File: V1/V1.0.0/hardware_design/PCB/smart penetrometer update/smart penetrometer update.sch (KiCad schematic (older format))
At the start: 34 parts, among them J1 XLR3_Switched, J2 Conn_01x11_Female, U2 DS3231M, U3 Battery_Input, U4 4023, U5 ADS1115IDGS, U6 3v3_Voltage_Regulator, U7 Solar_Input

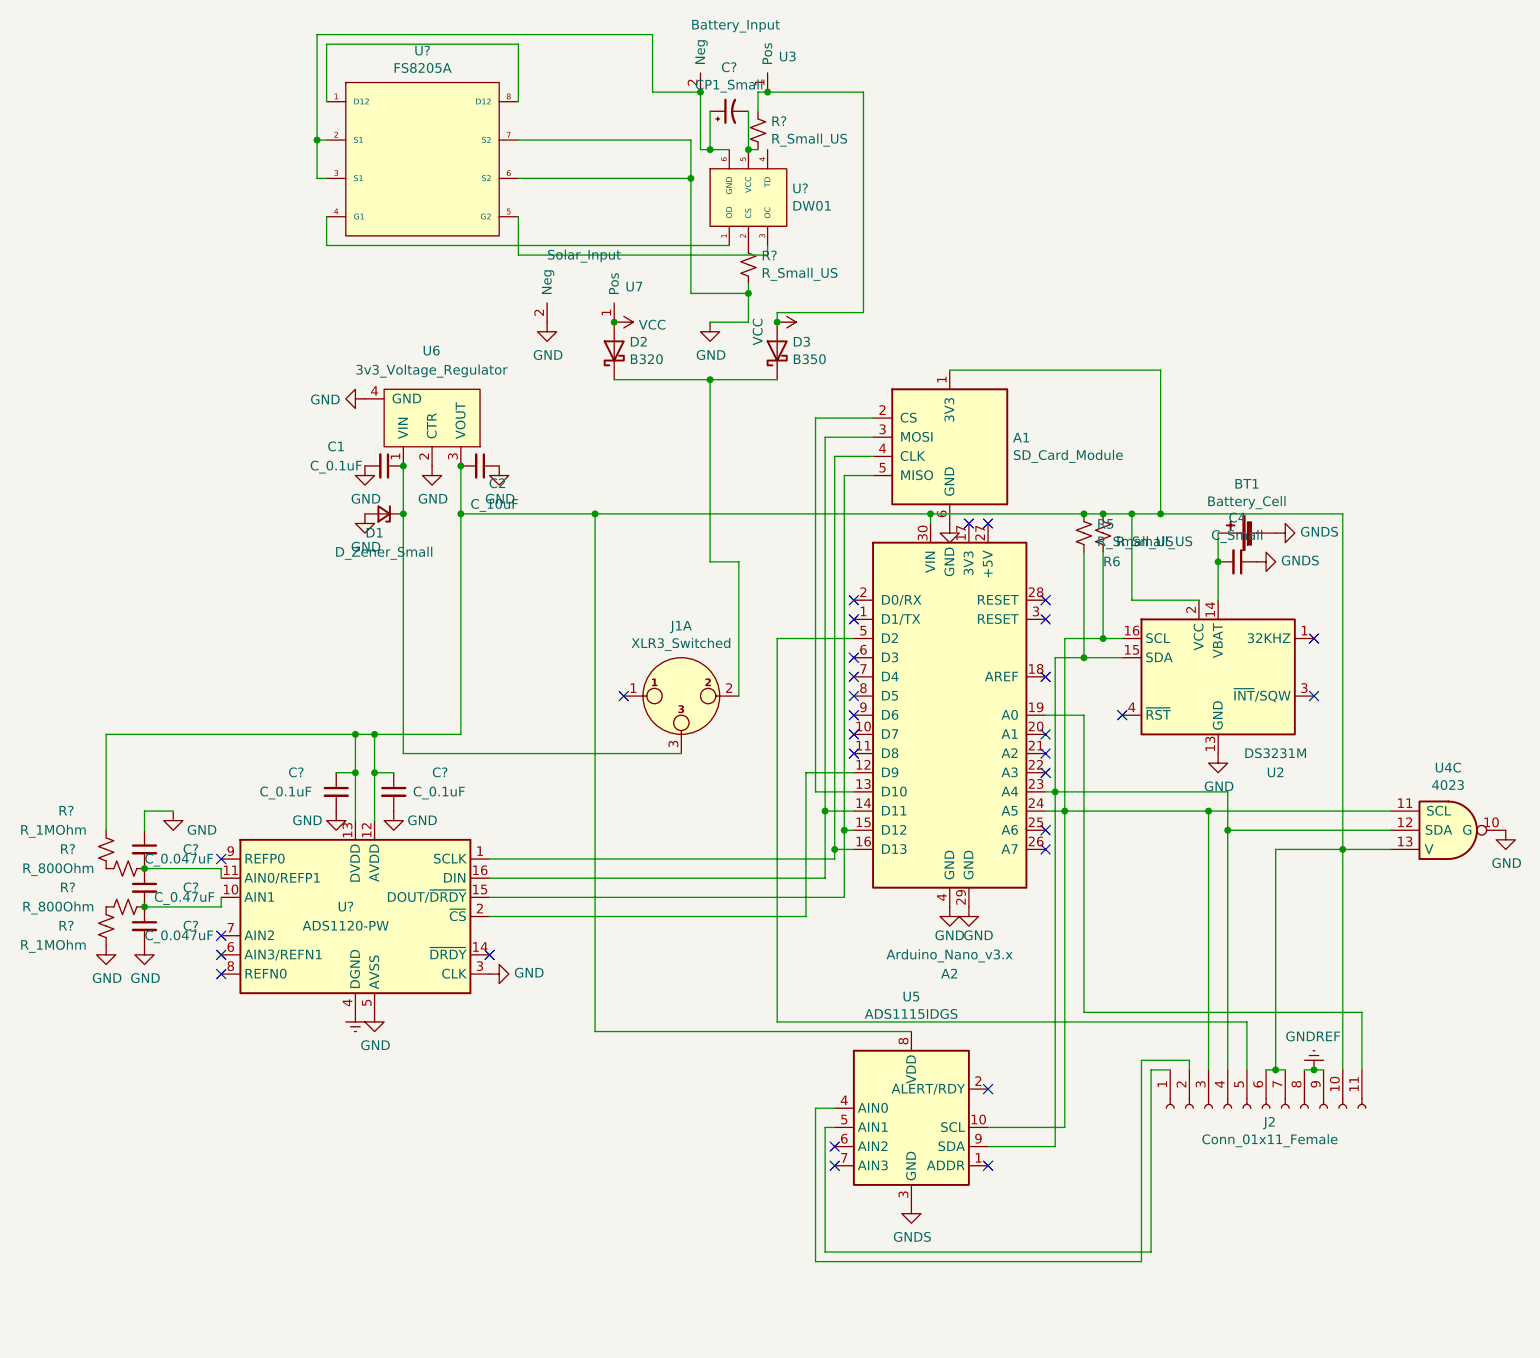
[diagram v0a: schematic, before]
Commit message: SCHEMATIC UPDAYE
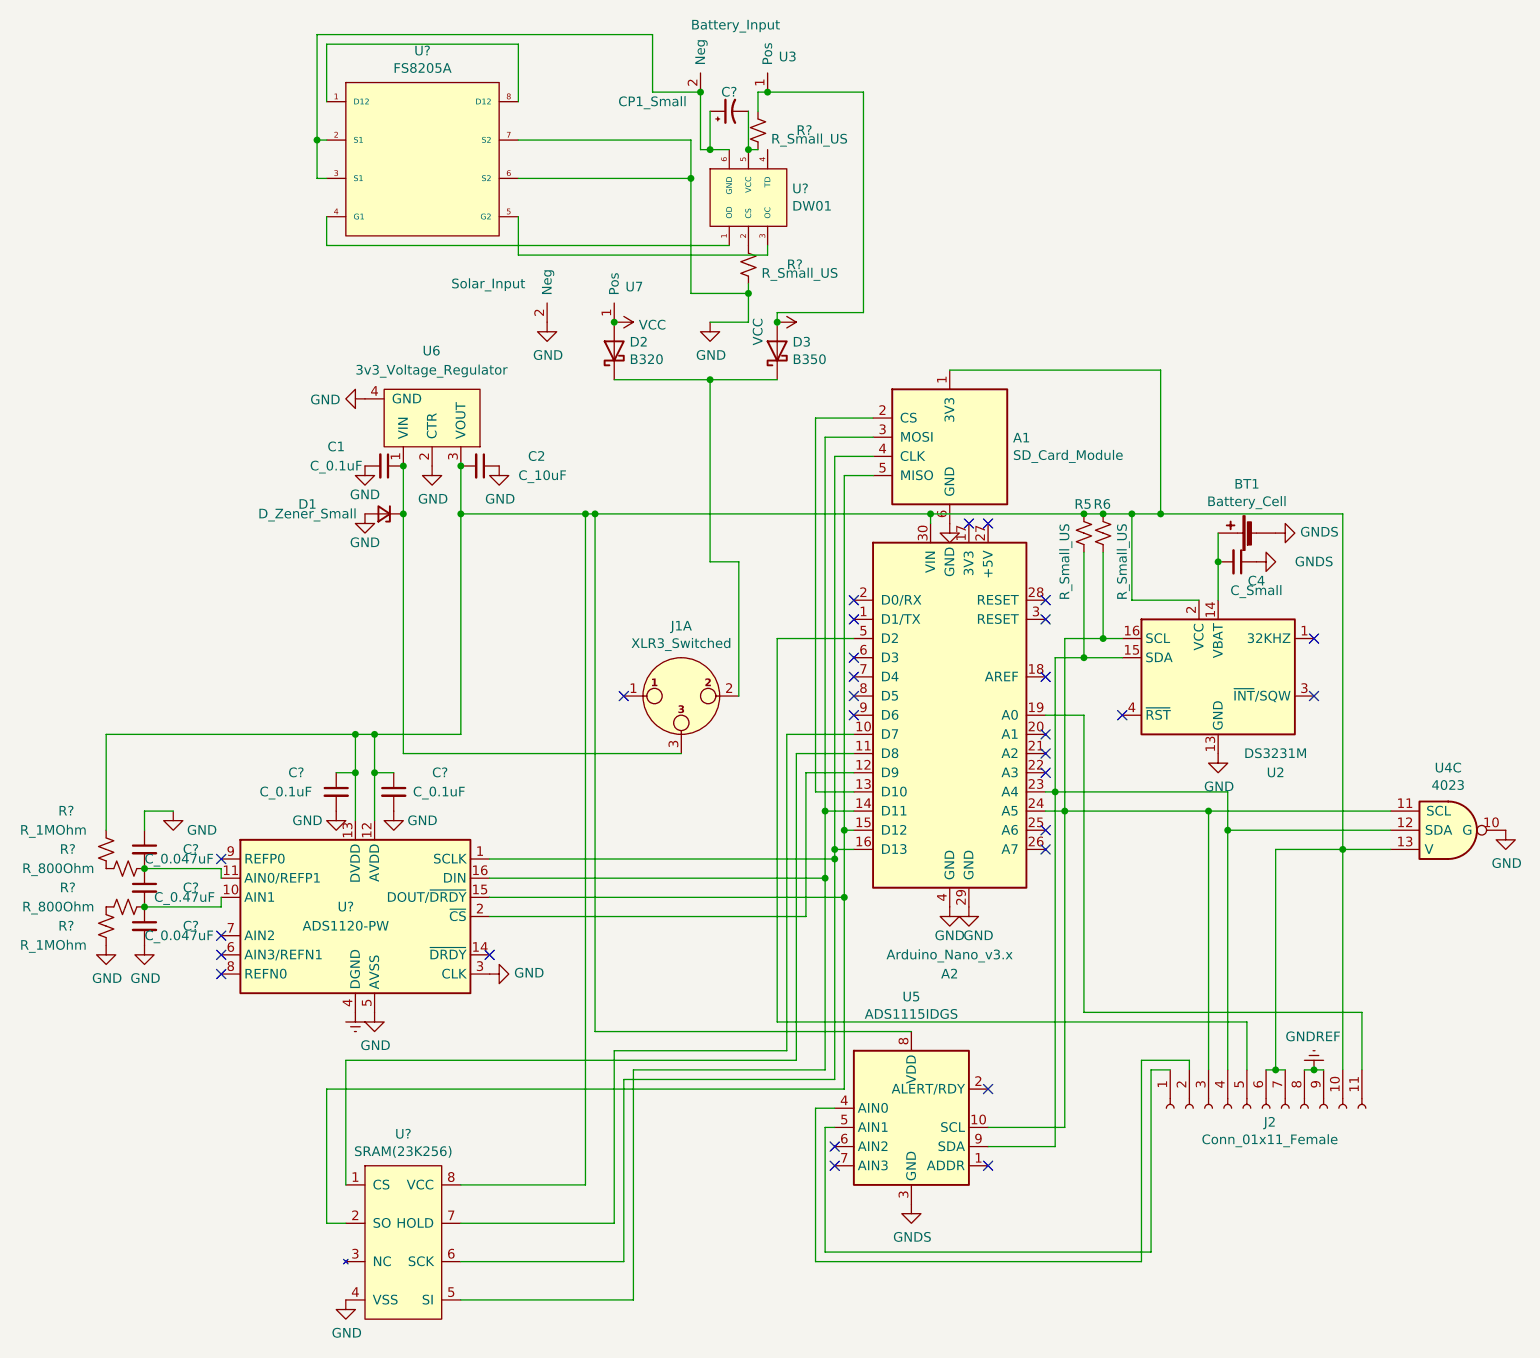
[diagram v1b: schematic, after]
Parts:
- added U?: SRAM(23K256), symbol smart-penetrometer-update-rescue:SRAM(23K256)
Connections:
- net GND: now also U?.4 (VSS)
- net at A2.10 (D7): now also U?.7 (HOLD)
- net at A2.11 (D8): now also U?.1 (CS)
- net at A1.3 (MOSI), A2.14 (D11), U?.16 (DIN): now also U?.5 (SI)
- net at A1.5 (MISO), A2.15 (D12), U?.15 (DOUT/~DRDY): now also U?.2 (SO)
- net at A1.4 (CLK), A2.16 (D13), U?.1 (SCLK): now also U?.6 (SCK)
- net at A1.1 (3V3), A2.30 (VIN), C2.2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: now also U?.8 (VCC)
- no-connect marks 31 -> 29
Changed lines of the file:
@@
 NoConn ~ 4850 4050
 NoConn ~ 4850 4150
-NoConn ~ 4850 4250
-NoConn ~ 4850 4350
 $Comp
 L smart-penetrometer-update-rescue:Battery_Input-kitest-kitest-rescue-smart-penetrometer-rescue U3
@@
 	1    0    0    -1
 $EndComp
-$Comp
-L Analog_ADC:ADS1115IDGS U5
-U 1 1 615B81A7
-P 5150 6300
-F 0 "U5" H 5150 6981 50  0000 C CNN
-F 1 "ADS1115IDGS" H 5150 6890 50  0000 C CNN
-F 2 "Package_SO:TSSOP-10_3x3mm_P0.5mm" H 5150 5800 50  0001 C CNN
-F 3 "http://www.ti.com/lit/ds/symlink/ads1113.pdf" H 5100 5400 50  0001 C CNN
-	1    5150 6300
-	1    0    0    -1
-$EndComp
 Wire Wire Line
 	5550 6300 5950 6300
@@
 U 1 1 6162D30F
 P 6050 3200
-F 0 "R5" H 6118 3246 50  0000 L CNN
-F 1 "R_Small_US" H 6118 3155 50  0000 L CNN
+F 0 "R5" H 6000 3350 50  0000 L CNN
+F 1 "R_Small_US" V 5950 2850 50  0000 L CNN
 F 2 "Resistor_SMD:R_1206_3216Metric" H 6050 3200 50  0001 C CNN
 F 3 "~" H 6050 3200 50  0001 C CNN
@@
 U 1 1 6162E2E0
 P 6150 3200
-F 0 "R6" H 6150 3050 50  0000 L CNN
-F 1 "R_Small_US" H 6218 3155 50  0000 L CNN
+F 0 "R6" H 6100 3350 50  0000 L CNN
+F 1 "R_Small_US" V 6250 2850 50  0000 L CNN
 F 2 "Resistor_SMD:R_1206_3216Metric" H 6150 3200 50  0001 C CNN
 F 3 "~" H 6150 3200 50  0001 C CNN
@@
 U 1 1 6163E9E6
 P 6850 3350
-F 0 "C4" V 6621 3350 50  0000 C CNN
-F 1 "C_Small" V 6712 3350 50  0000 C CNN
+F 0 "C4" V 6950 3450 50  0000 C CNN
+F 1 "C_Small" V 7000 3450 50  0000 C CNN
 F 2 "Capacitor_SMD:C_1206_3216Metric" H 6850 3350 50  0001 C CNN
 F 3 "~" H 6850 3350 50  0001 C CNN
@@
 P 6950 3350
 F 0 "#PWR011" H 6950 3100 50  0001 C CNN
-F 1 "GNDS" V 6955 3222 50  0000 R CNN
+F 1 "GNDS" V 6950 3150 50  0000 R CNN
 F 2 "" H 6950 3350 50  0001 C CNN
 F 3 "" H 6950 3350 50  0001 C CNN
@@
 U 1 1 61FFB484
 P 2900 2850
-F 0 "C2" V 2992 2896 50  0000 L CNN
-F 1 "C_10uF" V 3100 2800 50  0000 L CNN
+F 0 "C2" V 2850 3100 50  0000 L CNN
+F 1 "C_10uF" V 2950 3050 50  0000 L CNN
 F 2 "Capacitor_SMD:C_1206_3216Metric" H 2900 2850 50  0001 C CNN
 F 3 "~" H 2900 2850 50  0001 C CNN
@@
 U 1 1 62002596
 P 2400 3100
-F 0 "D1" H 2450 3200 50  0000 C CNN
-F 1 "D_Zener_Small" H 2400 3300 50  0000 C CNN
+F 0 "D1" H 2800 3050 50  0000 C CNN
+F 1 "D_Zener_Small" H 2800 3100 50  0000 C CNN
 F 2 "Diode_SMD:D_SMC" V 2400 3100 50  0001 C CNN
 F 3 "~" V 2400 3100 50  0001 C CNN
@@
 $EndComp
 Wire Wire Line
-	4700 6300 4700 6950
-Wire Wire Line
 	4700 6950 6400 6950
 Wire Wire Line
@@
 Wire Wire Line
 	4650 6200 4650 7000
-Wire Wire Line
-	4650 7000 6350 7000
 Wire Wire Line
 	6350 7000 6350 5950
@@
 P 3400 1950
 F 0 "U7" H 3658 1984 50  0000 L CNN
-F 1 "Solar_Input" H 3250 2150 50  0000 L CNN
+F 1 "Solar_Input" H 2750 2000 50  0000 L CNN
 F 2 "kitest:Battery_Input" H 3400 1950 50  0001 C CNN
 F 3 "" H 3400 1950 50  0001 C CNN
@@
 P 2300 3100
 F 0 "#PWR0106" H 2300 2850 50  0001 C CNN
-F 1 "GND" H 2305 2927 50  0000 C CNN
+F 1 "GND" H 2300 2950 50  0000 C CNN
 F 2 "" H 2300 3100 50  0001 C CNN
 F 3 "" H 2300 3100 50  0001 C CNN
@@
 P 2300 2850
 F 0 "#PWR0107" H 2300 2600 50  0001 C CNN
-F 1 "GND" H 2305 2677 50  0000 C CNN
+F 1 "GND" H 2300 2700 50  0000 C CNN
 F 2 "" H 2300 2850 50  0001 C CNN
 F 3 "" H 2300 2850 50  0001 C CNN
@@
 U 1 1 6280EF6A
 P 4300 1800
-F 0 "R?" H 4368 1846 50  0000 L CNN
+F 0 "R?" H 4500 1800 50  0000 L CNN
 F 1 "R_Small_US" H 4368 1755 50  0000 L CNN
 F 2 "" H 4300 1800 50  0001 C CNN
@@
 U 1 1 6280FAAE
 P 4350 1100
-F 0 "R?" H 4418 1146 50  0000 L CNN
+F 0 "R?" H 4550 1100 50  0000 L CNN
 F 1 "R_Small_US" H 4418 1055 50  0000 L CNN
 F 2 "" H 4350 1100 50  0001 C CNN
@@
 U 1 1 62819F8F
 P 4200 1000
-F 0 "C?" V 4428 1000 50  0000 C CNN
-F 1 "CP1_Small" V 4337 1000 50  0000 C CNN
+F 0 "C?" V 4300 1000 50  0000 C CNN
+F 1 "CP1_Small" V 4250 1400 50  0000 C CNN
 F 2 "" H 4200 1000 50  0001 C CNN
 F 3 "~" H 4200 1000 50  0001 C CNN
@@
 	2250 4250 2250 4450
 Wire Wire Line
-	2800 3100 3500 3100
+	2800 3100 3450 3100
 Connection ~ 2350 4250
 Connection ~ 2250 4450
@@
 	950  4250 950  4750
 Connection ~ 2250 4250
+$Comp
+L smart-penetrometer-update-rescue:SRAM(23K256) U?
+U 1 1 62EB656F
+P 2500 6900
+F 0 "U?" H 2500 7465 50  0000 C CNN
+F 1 "SRAM(23K256)" H 2500 7374 50  0000 C CNN
+F 2 "" H 2500 6900 50  0001 C CNN
+F 3 "" H 2500 6900 50  0001 C CNN
+	1    2500 6900
+	1    0    0    -1
+$EndComp
+Wire Wire Line
+	2800 6600 3450 6600
+Wire Wire Line
+	3450 6600 3450 3100
+Connection ~ 3450 3100
+Wire Wire Line
+	3450 3100 3500 3100
+$Comp
+L power:GND #PWR?
+U 1 1 62FCEB65
+P 2200 7200
+F 0 "#PWR?" H 2200 6950 50  0001 C CNN
+F 1 "GND" H 2205 7027 50  0000 C CNN
+F 2 "" H 2200 7200 50  0001 C CNN
+F 3 "" H 2200 7200 50  0001 C CNN
+	1    2200 7200
+	1    0    0    -1
+$EndComp
+$Comp
+L Analog_ADC:ADS1115IDGS U5
+U 1 1 615B81A7
+P 5150 6300
+F 0 "U5" H 5150 6981 50  0000 C CNN
+F 1 "ADS1115IDGS" H 5150 6890 50  0000 C CNN
+F 2 "Package_SO:TSSOP-10_3x3mm_P0.5mm" H 5150 5800 50  0001 C CNN
+F 3 "http://www.ti.com/lit/ds/symlink/ads1113.pdf" H 5100 5400 50  0001 C CNN
+	1    5150 6300
+	1    0    0    -1
+$EndComp
+Wire Wire Line
+	4700 6300 4700 6950
+Wire Wire Line
+	4650 7000 6350 7000
+Wire Wire Line
+	4750 4900 4750 6050
+Wire Wire Line
+	4750 6050 3650 6050
+Wire Wire Line
+	3650 6050 3650 7000
+Wire Wire Line
+	3650 7000 2800 7000
+Connection ~ 4750 4900
+Wire Wire Line
+	4700 5000 4700 6000
+Wire Wire Line
+	4700 6000 3700 6000
+Wire Wire Line
+	3700 6000 3700 7200
+Wire Wire Line
+	3700 7200 2800 7200
+Connection ~ 4700 5000
+Wire Wire Line
+	4800 5100 4800 6100
+Wire Wire Line
+	4800 6100 2100 6100
+Wire Wire Line
+	2100 6100 2100 6800
+Wire Wire Line
+	2100 6800 2200 6800
+Connection ~ 4800 5100
+Wire Wire Line
+	2200 6600 2200 5950
+Wire Wire Line
+	2200 5950 4550 5950
+Wire Wire Line
+	4550 5950 4550 4350
+Wire Wire Line
+	4550 4350 4850 4350
+Wire Wire Line
+	2800 6800 3600 6800
+Wire Wire Line
+	3600 6800 3600 5900
+Wire Wire Line
+	3600 5900 4500 5900
+Wire Wire Line
+	4500 5900 4500 4250
+Wire Wire Line
+	4500 4250 4850 4250
 $EndSCHEMATC
